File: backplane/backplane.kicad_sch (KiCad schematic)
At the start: 13 parts, among them U1 PT4115

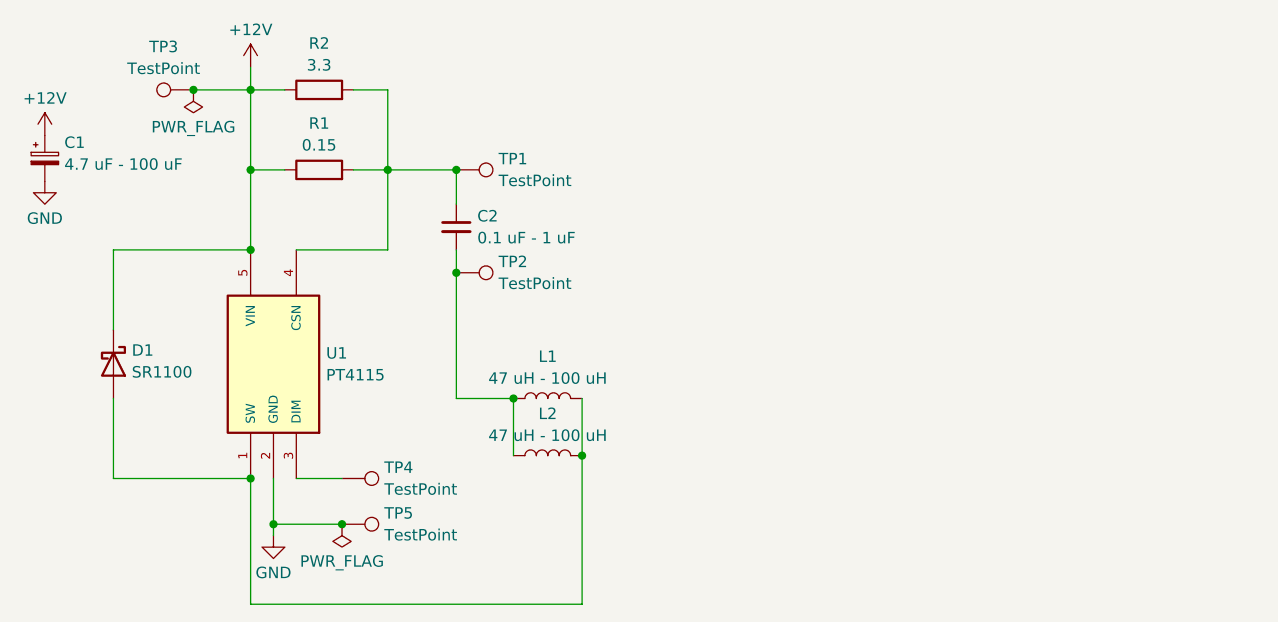
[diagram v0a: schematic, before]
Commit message: Backplane work
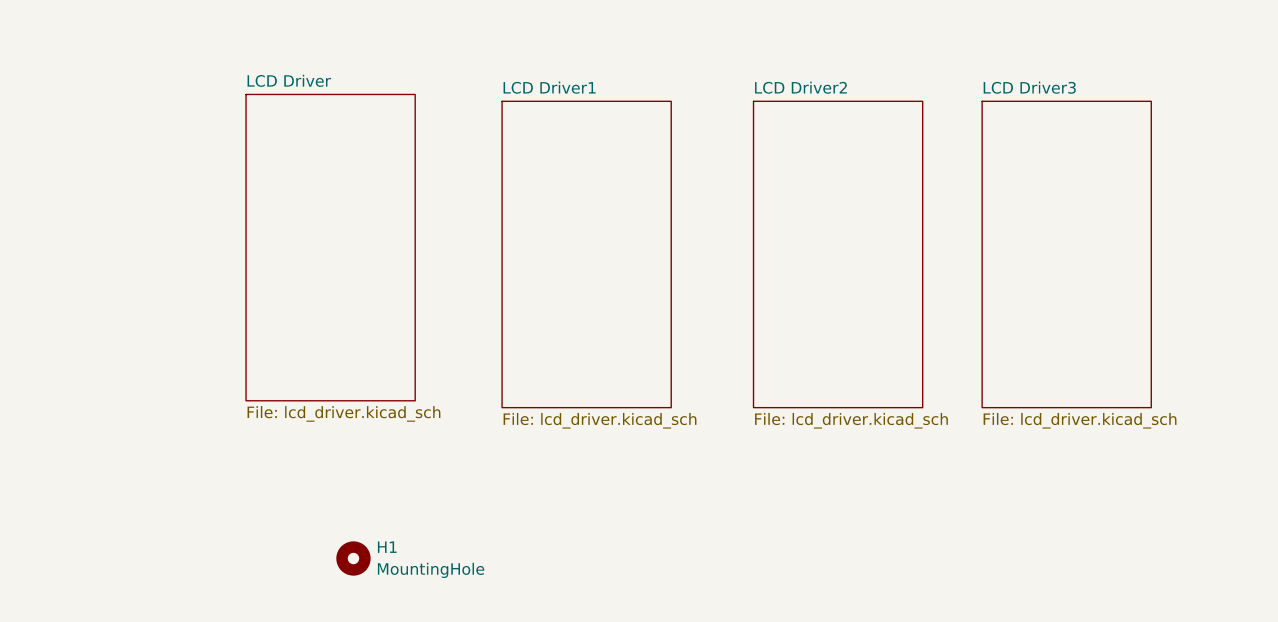
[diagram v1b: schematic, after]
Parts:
- removed C1: 4.7 uF - 100 uF, Capacitor_THT:CP_Radial_D6.3mm_P2.50mm, symbol Device:C_Polarized_Small
- removed C2: 0.1 uF - 1 uF, Capacitor_THT:C_Disc_D6.0mm_W2.5mm_P5.00mm, symbol Device:C_Small
- removed D1: SR1100, Diode_THT:D_DO-35_SOD27_P7.62mm_Horizontal, symbol Device:D_Schottky
- removed L1, L2: 47 uH - 100 uH, Inductor_THT:L_Axial_L9.5mm_D4.0mm_P12.70mm_Horizontal_Fastron_SMCC, symbol Device:L
- removed R1: 0.15, Resistor_THT:R_Axial_DIN0207_L6.3mm_D2.5mm_P7.62mm_Horizontal, symbol Device:R
- removed R2: 3.3, Resistor_THT:R_Axial_DIN0207_L6.3mm_D2.5mm_P7.62mm_Horizontal, symbol Device:R
- removed TP1, TP2, TP3, TP4, TP5: TestPoint, TestPoint:TestPoint_THTPad_D1.5mm_Drill0.7mm, symbol Connector:TestPoint
- removed U1: PT4115, Package_TO_SOT_SMD:SOT-89-5, symbol misc:PT4115
- added H1: MountingHole, MountingHole:MountingHole_2.2mm_M2, symbol Mechanical:MountingHole
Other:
- added sheet LCD Driver (lcd_driver.kicad_sch)
- added sheet LCD Driver1 (lcd_driver.kicad_sch)
- added sheet LCD Driver2 (lcd_driver.kicad_sch)
- added sheet LCD Driver3 (lcd_driver.kicad_sch)
